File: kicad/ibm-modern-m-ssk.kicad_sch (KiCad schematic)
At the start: 55 parts, among them J1 TF38-24S-0.5SV(830), J2 S2B-PH-SM4-TB(LF)(SN), J3 Conn_02x06_Odd_Even, J4 Conn_01x04_Pin, J5 726386-2, Q1 DMP2123LQ, SW90 SW_Push, U2 BQ24075RGTR, U3 XC6220B331ER-G, U4 LC709203FXE-03MH, Y1 32MHz, Y2 32.768 kHz

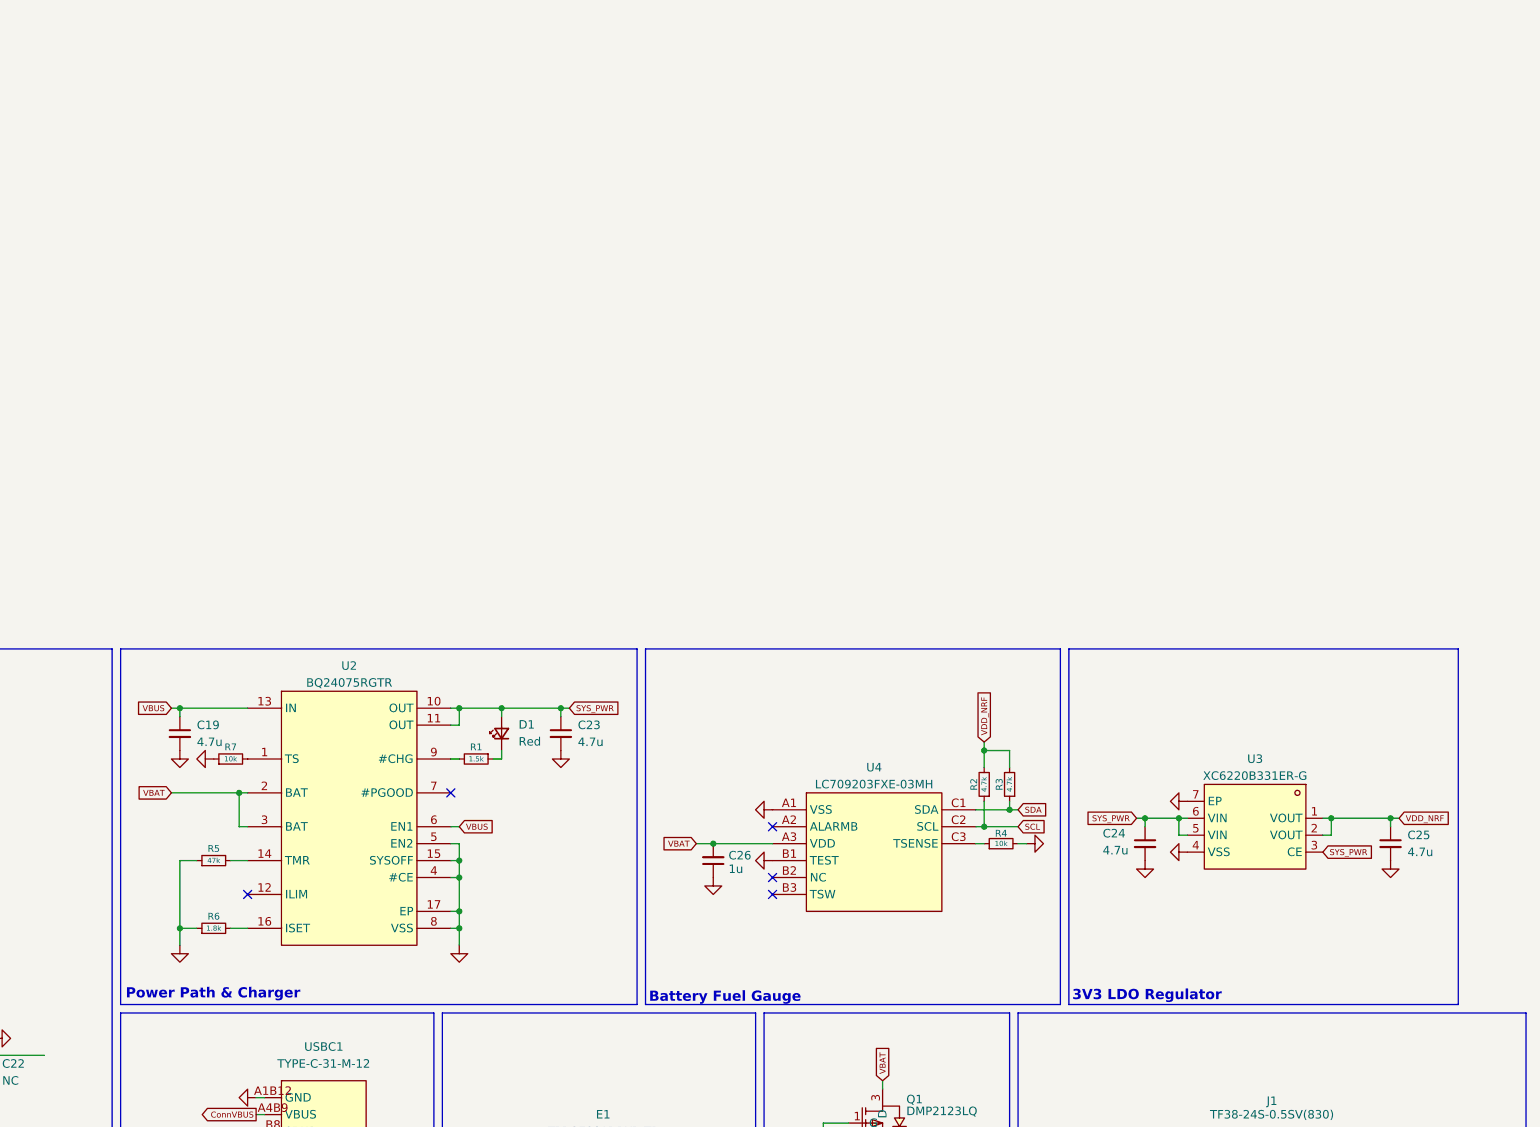
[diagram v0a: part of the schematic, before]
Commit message: update lolololololololo
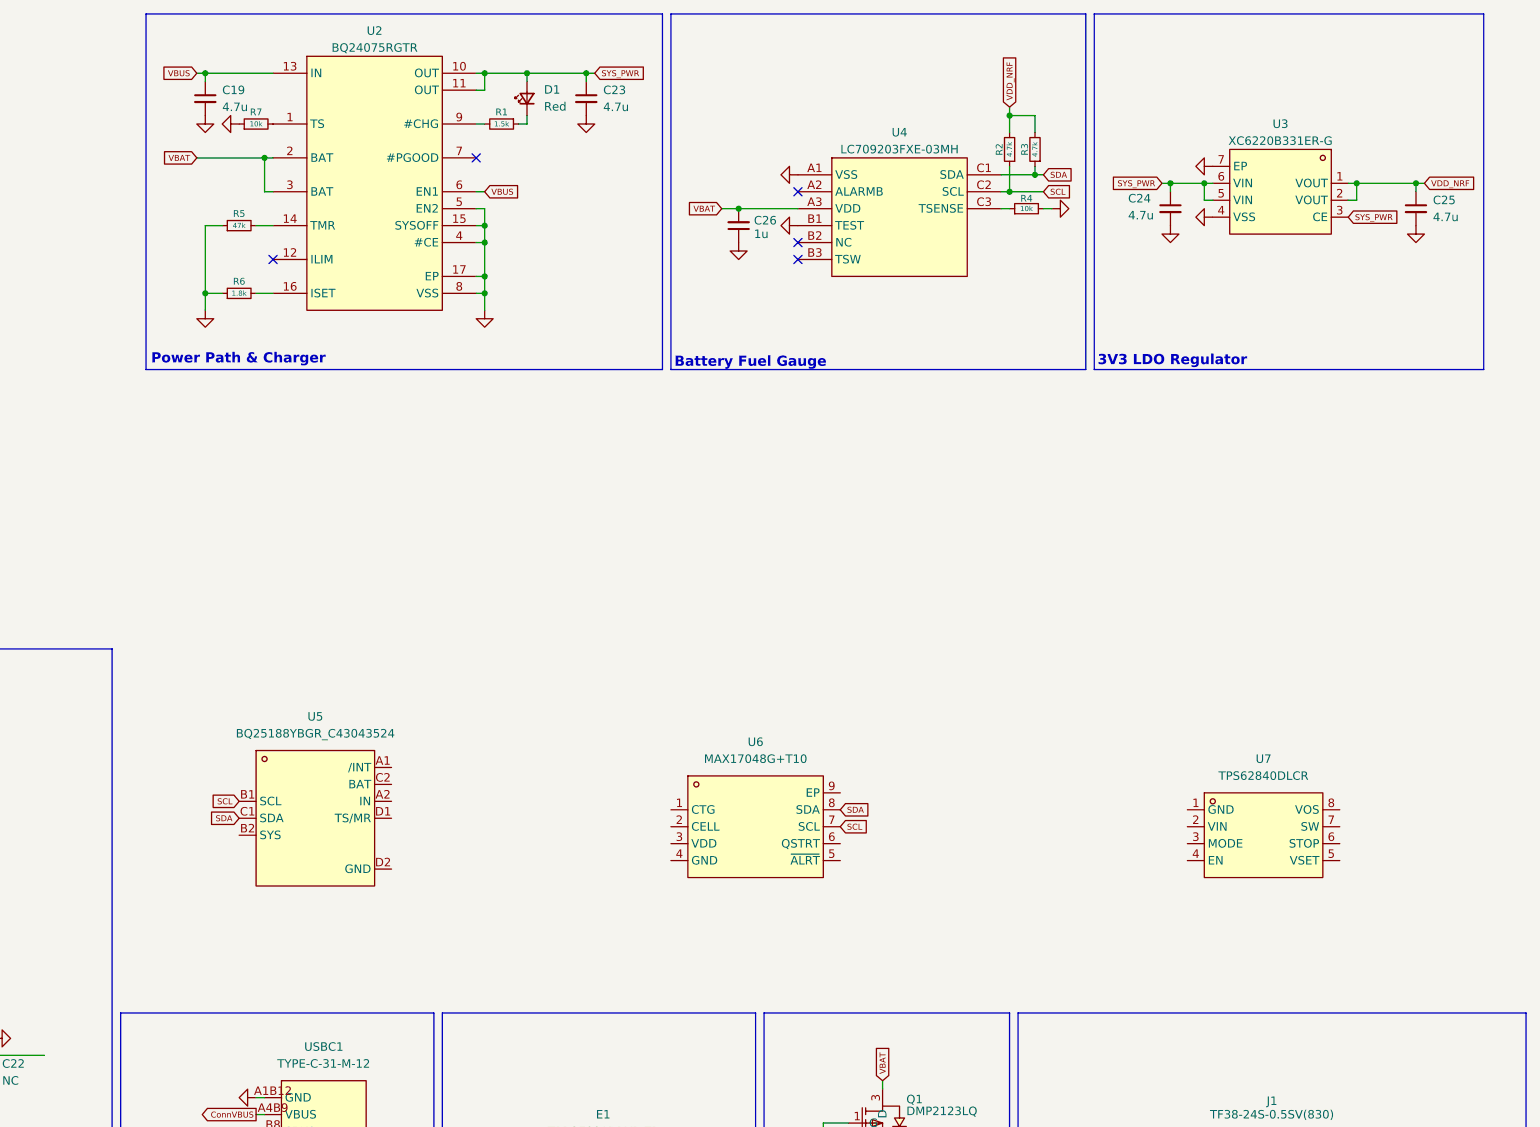
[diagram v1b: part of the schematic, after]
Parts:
- added U5: BQ25188YBGR_C43043524, easyeda2kicad:WCSP-8_L1.6-W1.0-P0.40-TL_IS31FL3194-CLS2, symbol easyeda2kicad:BQ25188YBGR_C43043524
- added U6: MAX17048G+T10, easyeda2kicad:TDFN-8_L2.0-W2.0-P0.50-BL-EP1.2, symbol easyeda2kicad:MAX17048G+T10
- added U7: TPS62840DLCR, easyeda2kicad:VSON-8_L2.0-W1.5-P0.50-BL, symbol easyeda2kicad:TPS62840DLCR
- U1: value ~ -> NRF52840
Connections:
- net SCL: now also U5.B1 (SCL), U6.7 (SCL)
- net SDA: now also U5.C1 (SDA), U6.8 (SDA)
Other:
- moved on the sheet: C19, C23, C24, C25, C26, D1, R1, R2, R3, R4, R5, R6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
